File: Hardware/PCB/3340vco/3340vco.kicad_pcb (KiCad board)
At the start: 2 copper layers, 214 x 172 mm, 140 parts, among them J1 Conn_02x04_Odd_Even, J10 AudioJack2, J11 AudioJack2, J12 AudioJack2, J13 AudioJack2, J14 AudioJack2, J15 AudioJack2, J16 3_pin_Molex_connector, J17 Conn_01x03, J18 Conn_01x03, J19 Conn_01x03, J2 Conn_01x06, J20 Conn_01x03, J21 Conn_01x03, J22 Conn_01x03, J23 Conn_01x07, J24 Conn_01x07, J3 3_pin_Molex_header, J4 Conn_01x06, J5 Synth_power_2x5, J6 AudioJack2, J7 AudioJack2, J8 AudioJack2, J9 AudioJack2, Q1 2N3904, Q2 2N3904, SW1 SW_SPDT_MSM, SW2 SW_Rotary12, U1 TL074, U2 AS3340A, U3 TL072, U4 TL431LP, U5 L79L05_TO92, U6 TL074

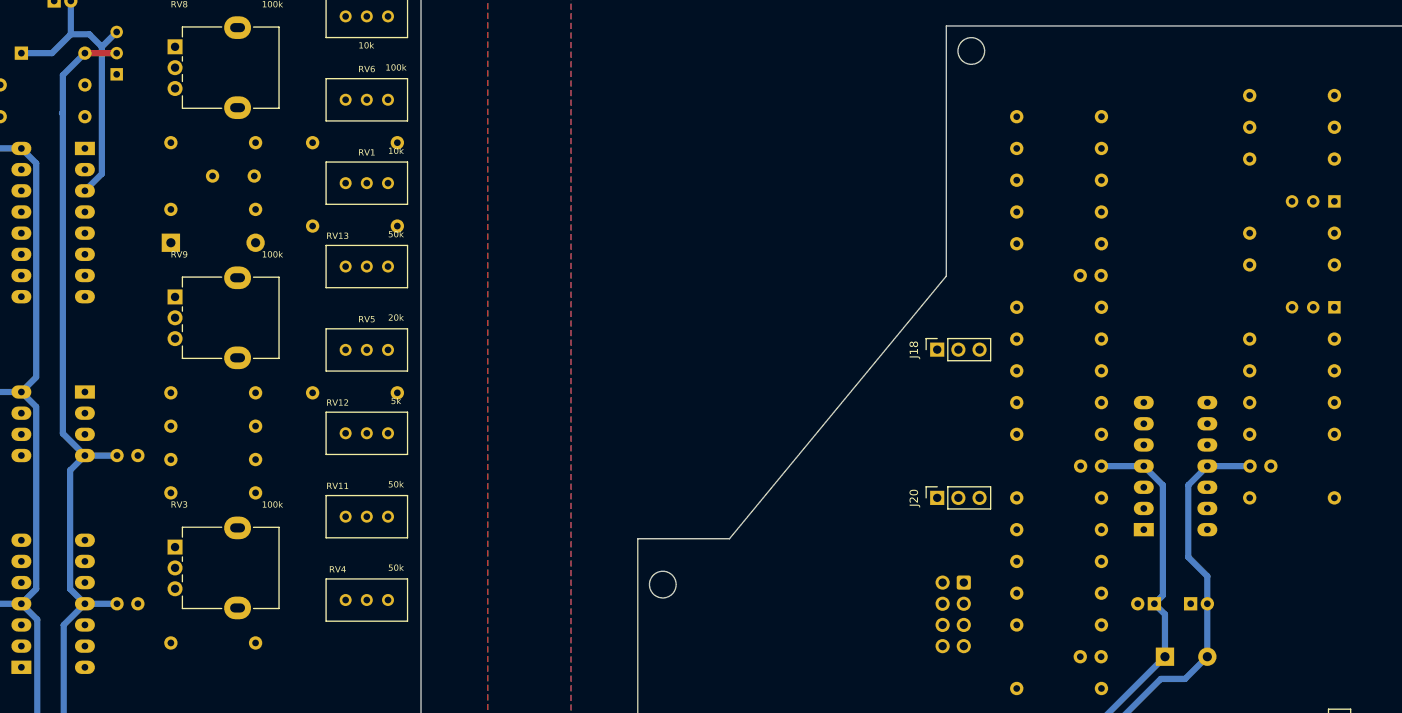
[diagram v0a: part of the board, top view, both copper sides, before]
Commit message: Fix label
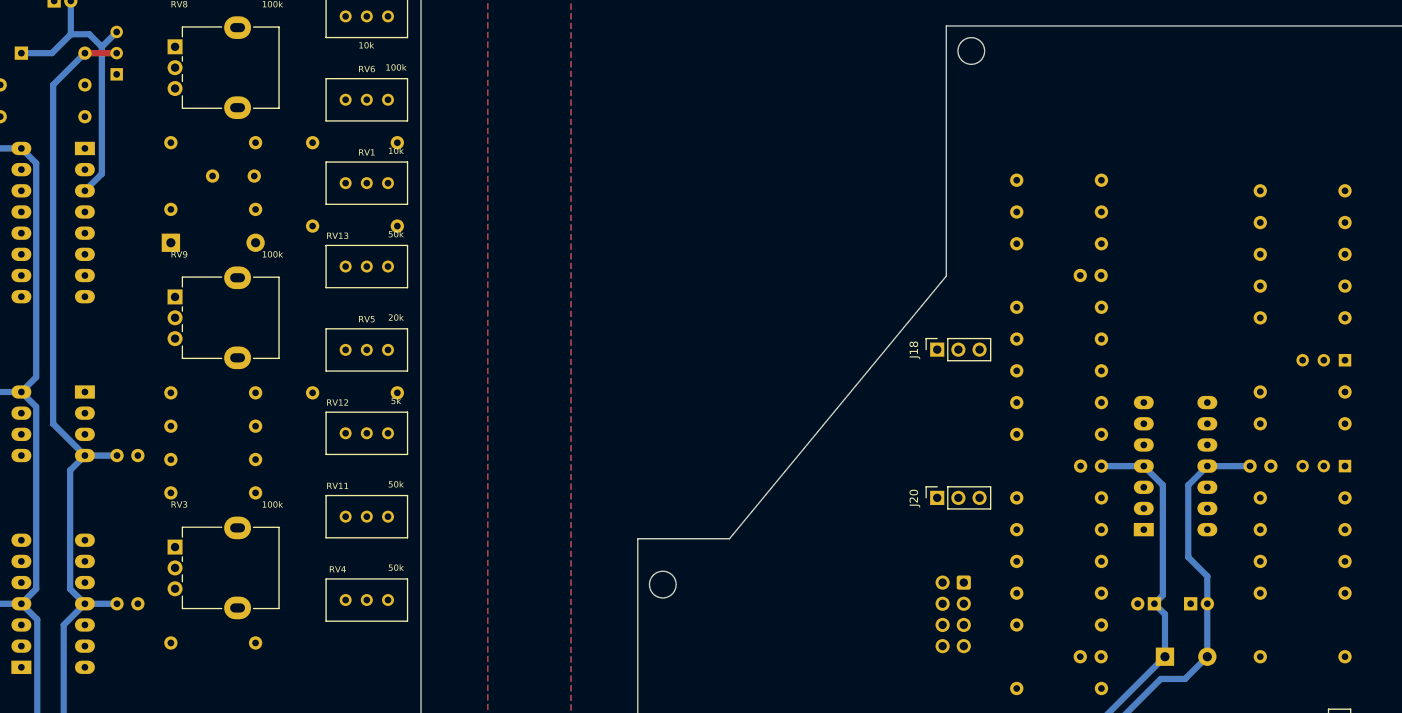
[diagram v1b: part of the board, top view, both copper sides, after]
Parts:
- moved R47 30.5 mm to (327.7, 68.6)
- moved R44 30.5 mm to (327.7, 64.8)
- moved R38 19.1 mm to (327.7, 88.9)
- moved Q1 19.1 mm to (337.8, 97.8)
- moved R39 19.1 mm to (337.8, 120.7)
- moved R35 19.1 mm to (337.8, 80.0)
- moved R61 19.1 mm to (337.8, 76.2)
- moved R37 19.1 mm to (327.7, 105.4)
- moved R59 19.1 mm to (327.7, 72.4)
- moved R60 19.1 mm to (327.7, 92.7)
- moved R63 19.1 mm to (327.7, 113.0)
- moved Q2 19.1 mm to (337.8, 85.1)
- moved R36 19.1 mm to (337.8, 101.6)
- moved R62 19.1 mm to (337.8, 109.2)
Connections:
- RV4 pad 3: SIN_S_CCW -> SIN_S_CW
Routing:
- net -12V_P: track 98.9 -> 99.7 mm

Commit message: Revise power ports
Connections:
- C10 pad 2: -12V_P -> -12V
- C11 pad 1: +12V -> +12V_1
- C12 pad 2: -12V -> -12V_1
- C14 pad 1: +12V -> +12V_1
- C15 pad 2: -12V -> -12V_1
- C3 pad 1: +12V_P -> +12V
- C6 pad 1: +12V_P -> +12V
- C7 pad 2: -12V_P -> -12V
- C9 pad 1: +12V_P -> +12V
- D1 pad 1: +12V -> +12V_1
- D2 pad 2: -12V -> -12V_1
- D3 pad 2: -12V_P -> -12V
- J21 pad 2: +12V_P -> +12V
- J21 pad 3: -12V_P -> -12V
- J22 pad 2: +12V -> +12V_1
- J22 pad 3: -12V -> -12V_1
- R13 pad 1: +12V_P -> +12V
- R19 pad 2: +12V_P -> +12V
- R26 pad 2: +12V_P -> +12V
- R37 pad 1: +12V -> +12V_1
- R44 pad 2: +12V -> +12V_1
- R45 pad 2: +12V -> +12V_1
- R46 pad 2: +12V -> +12V_1
- R59 pad 1: +12V -> +12V_1
- R60 pad 1: -12V -> -12V_1
- R8 pad 1: Net-(R8-Pad1) -> Net-(R10-Pad2)
- RV8 pad 1: -12V_P -> -12V
- RV8 pad 3: +12V_P -> +12V
- U1 pad 11: -12V_P -> -12V
- U1 pad 4: +12V_P -> +12V
- U2 pad 16: +12V_P -> +12V
- U3 pad 4: -12V_P -> -12V
- U3 pad 8: +12V_P -> +12V
- U5 pad 2: -12V_P -> -12V
- U6 pad 11: -12V -> -12V_1
- U6 pad 4: +12V -> +12V_1
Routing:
- net +12V_P: track 102.6 -> 0.00 mm
- net -12V_P: track 99.7 -> 0.00 mm
- net -12V_1: track 0.00 -> 51.9 mm
- net +12V_1: track 0.00 -> 51.8 mm
- net +12V: track 51.8 -> 102.6 mm
- net -12V: track 51.9 -> 99.7 mm
